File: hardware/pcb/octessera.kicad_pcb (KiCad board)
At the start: 2 copper layers, 107.2 x 127 mm, 11 parts, among them J1 NeoTrellis_Conn, SW1 RotaryEncoder_Switch, SW2 RotaryEncoder_Switch, SW3 RotaryEncoder_Switch, SW4 RotaryEncoder_Switch, U1 Raspberry Zero 2 W, U2 SSD1351, U3 USB-C, U4 PCM5102a, U5 NeoKey

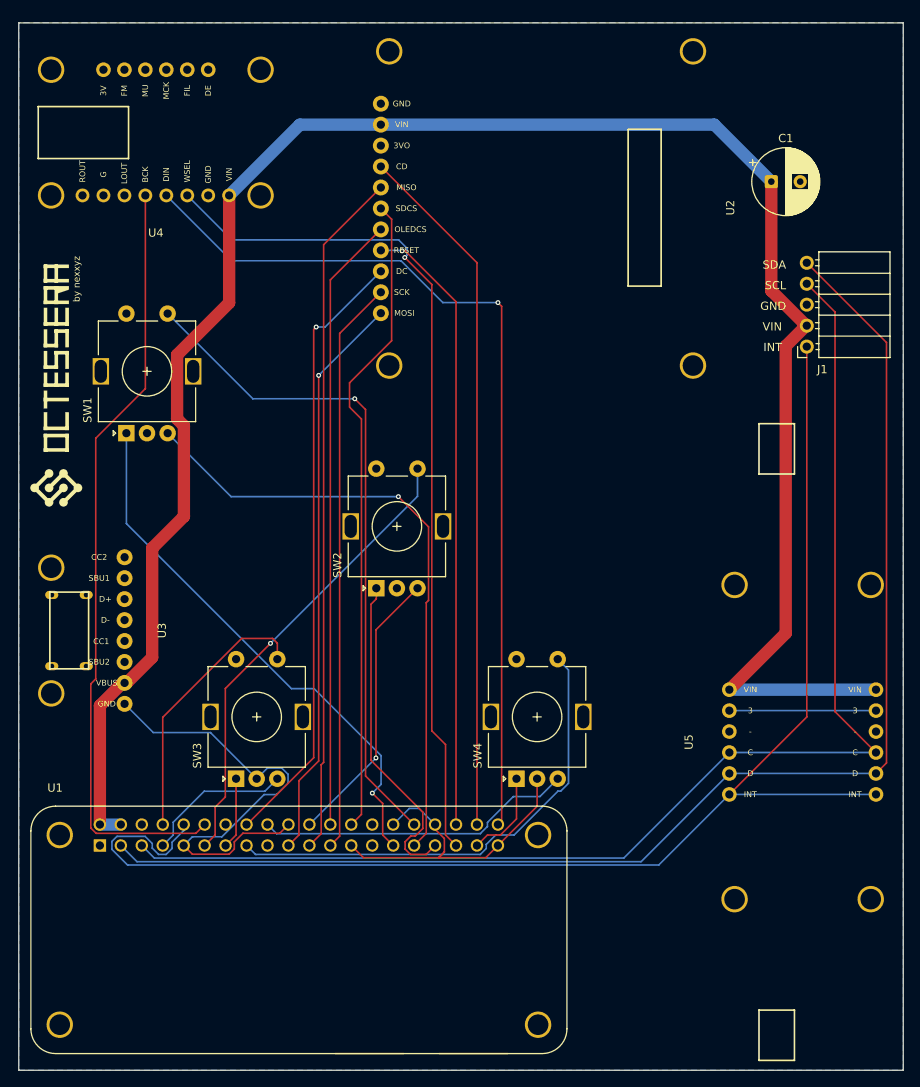
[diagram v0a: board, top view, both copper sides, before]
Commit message: Update PCB protection and fabrication outputs
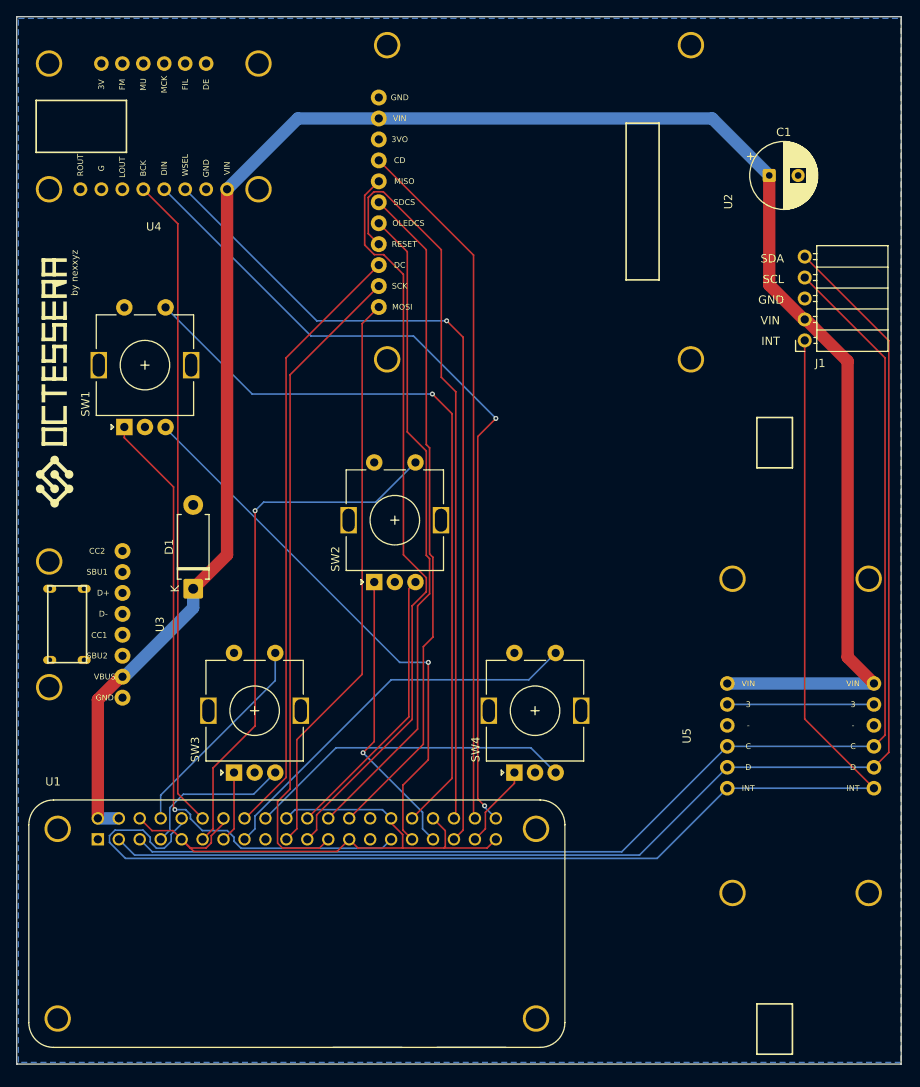
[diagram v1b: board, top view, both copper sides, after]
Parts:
- added D1: SA5.0A, Diode_THT:D_DO-15_P10.16mm_Horizontal, F.Cu at (35.4, 83.4)
- moved C1 0.79 mm to (105.2, 33.2)
- moved J1 0.79 mm to (121.0, 43.2)
- moved SW1 0.79 mm to (27.1, 63.8)
- moved SW2 0.79 mm to (57.4, 82.5)
- moved SW3 0.79 mm to (40.4, 105.7)
- moved SW4 0.79 mm to (74.3, 105.7)
- moved U1 0.79 mm to (48.0, 124.0)
- moved U2 0.79 mm to (98.3, 14.9)
- moved U3 0.79 mm to (29.4, 77.5)
- moved U4 0.79 mm to (45.9, 37.5)
- moved U5 0.79 mm to (98.3, 139.3)
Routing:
- net GND: track 97.9 -> 76.2 mm
- net Net-(U1-GPIO18/GPIO_GEN1): track 94.0 -> 79.3 mm
- net Net-(U1-GPIO16): track 75.1 -> 88.0 mm, vias 1 -> 0
- net Net-(U1-GPIO5): track 65.9 -> 78.1 mm
- net Net-(U1-GPIO22/GPIO_GEN3): track 58.9 -> 48.0 mm
- net Net-(U1-GPIO11/SPI_SCLK): track 69.6 -> 79.5 mm
- net Net-(U1-GPIO12): track 81.6 -> 91.2 mm
- net Net-(U1-GPIO6): track 75.7 -> 67.0 mm
- net Net-(U1-GPIO17/GPIO_GEN0): track 56.4 -> 64.3 mm
- net Net-(U1-GPIO14/TXD0): track 33.0 -> 25.8 mm
- net Net-(U1-GPIO21): track 109.3 -> 102.0 mm, vias 1 -> 2
- net Net-(U1-GPIO9/SPI_MISO): track 83.4 -> 90.2 mm
- net Net-(U1-GPIO8/SPI_~{CE0}): track 74.7 -> 79.8 mm
- net Net-(U1-GPIO13): track 40.0 -> 35.3 mm, vias 0 -> 1
- net Net-(U1-GPIO7/SPI_~{CE1}): track 78.5 -> 81.6 mm
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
